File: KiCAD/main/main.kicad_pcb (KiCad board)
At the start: 2 copper layers, 21.9 x 63.9 mm, 45 parts, among them J1 USB_C_Receptacle_USB2.0_14P, J2 Conn_Coaxial, J3 Conn_01x07_Socket, SW1 SW_SPDT, U1 SX1262IMLTRT, U2 TP4056-42-ESOP8, U3 BGS12P2L, U4 ESP32-S3-MINI-1, U6 MIC5219-3.3YMM, U7 CH340X

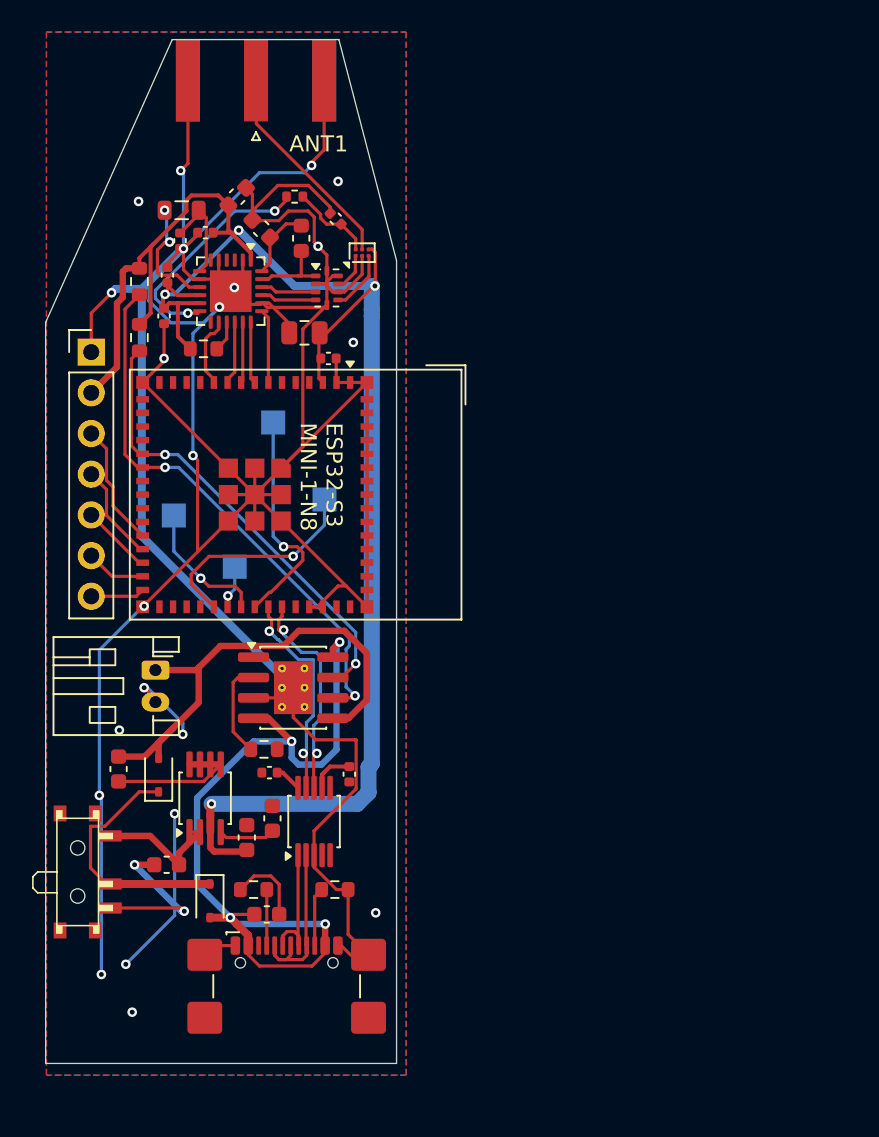
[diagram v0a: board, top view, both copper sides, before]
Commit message: Rev 3 done!
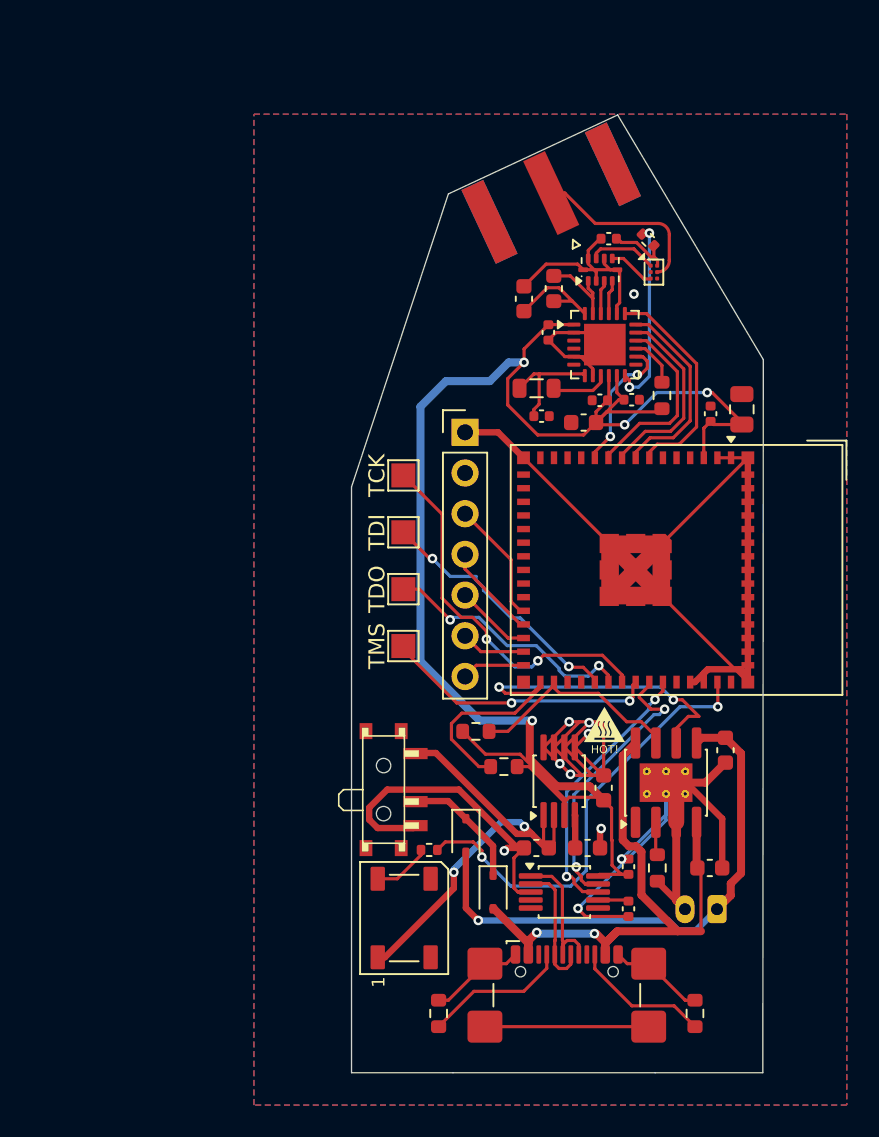
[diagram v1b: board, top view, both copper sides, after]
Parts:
- removed the G*** at (98.8, 76.4)
- removed TP1, TP2, TP3, TP4: TestPoint, TestPoint:TestPoint_Pad_1.5x1.5mm
- added D3: WS2812B, LED_SMD:LED_WS2812B_PLCC4_5.0x5.0mm_P3.2mm, F.Cu at (107.4, 85.3)
- added G***: LOGO, customlib:Hot_Sym, F.Cu at (119.9, 73.2)
- added R18: 450R, Resistor_SMD:R_0402_1005Metric, F.Cu at (108.9, 81.1)
- added TCK: TestPoint, TestPoint:TestPoint_Pad_1.5x1.5mm, F.Cu at (107.3, 57.7)
- added TDI: TestPoint, TestPoint:TestPoint_Pad_1.5x1.5mm, F.Cu at (107.3, 61.2)
- added TDO: TestPoint, TestPoint:TestPoint_Pad_1.5x1.5mm, F.Cu at (107.3, 64.8)
- added TMS: TestPoint, TestPoint:TestPoint_Pad_1.5x1.5mm, F.Cu at (107.3, 68.3)
- BT1: moved to B.Cu
- moved BT1 38.1 mm to (126.9, 84.8), turned to 180 degrees
- moved C16 37.9 mm to (127.4, 74.8)
- moved R9 37.9 mm to (113.6, 75.9), turned to 0 degrees
- moved R10 32.3 mm to (111.8, 73.7), turned to 180 degrees
- moved C10 29.7 mm to (121.6, 53.0), turned to 0 degrees
- moved R4 28.8 mm to (123.5, 52.7), turned to 90 degrees
- moved C7 28.1 mm to (119.6, 53.0), turned to 180 degrees
- moved C15 27.8 mm to (126.5, 82.2)
- moved C4 27.7 mm to (128.4, 53.6), turned to -90 degrees
- moved C14 25.8 mm to (118.6, 54.4), turned to 0 degrees
- moved R7 25.6 mm to (123.2, 82.2), turned to -90 degrees
- moved C11 25.1 mm to (116.0, 54.0), turned to 180 degrees
- moved L1 24.8 mm to (115.6, 52.3), turned to 0 degrees
- moved U4 24.2 mm to (124.4, 63.6)
- moved C3 24.1 mm to (126.5, 53.9), turned to -90 degrees
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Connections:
- net Net-(SW1-A) renamed +5V
- net V- renamed GND
- C10 pad 1: VCC -> +3.3V
- C14 pad 2: VCC -> +3.3V
- C17 pad 2: VCC -> +3.3V
- C18 pad 2: VCC -> +3.3V
- C2 pad 2: VCC -> +3.3V
- C3 pad 2: VCC -> +3.3V
- C4 pad 2: VCC -> +3.3V
- C6 pad 1: VCC -> +3.3V
- C7 pad 1: VCC -> +3.3V
- R10 pad 2: VCC -> +3.3V
- R4 pad 1: VCC -> +3.3V
- R9 pad 2: VCC -> +3.3V
- U1 pad 1: VCC -> +3.3V
- U1 pad 10: VCC -> +3.3V
- U1 pad 11: VCC -> +3.3V
- U3 pad 4: VCC -> +3.3V
- U4 pad 12: unconnected-(U4-IO8-Pad12) -> SDA
- U4 pad 13: unconnected-(U4-IO9-Pad13) -> SCL
- U4 pad 14: unconnected-(U4-IO10-Pad14) -> ENC_PHS_B
- U4 pad 15: unconnected-(U4-IO11-Pad15) -> ENC_PHS_A
- U4 pad 16: unconnected-(U4-IO12-Pad16) -> SEL
- U4 pad 17: unconnected-(U4-IO13-Pad17) -> PWR
- U4 pad 20: ~{CHRG} -> unconnected-(U4-IO16-Pad20)
- U4 pad 21: ~{STDBY} -> unconnected-(U4-IO17-Pad21)
- U4 pad 3: VCC -> +3.3V
- U4 pad 31: unconnected-(U4-IO35-Pad31) -> ~{STDBY}
- U4 pad 32: unconnected-(U4-IO36-Pad32) -> ~{CHRG}
- U4 pad 44: unconnected-(U4-IO46-Pad44) -> NEOPXL_D
- U6 pad 3: VCC -> +3.3V
- U7 pad 10: VCC -> +3.3V
- U7 pad 7: VCC -> +3.3V
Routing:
- net VCC: track 118.4 -> 0.00 mm, vias 4 -> 0
- net +3.3V: track 0.00 -> 107.8 mm, vias 0 -> 4
- net GND: track 313.6 -> 210.2 mm, vias 24 -> 10
- net NEOPXL_D: track 0.00 -> 27.8 mm, vias 0 -> 2
- net +5V: track 8.50 -> 29.1 mm, vias 0 -> 2
- net TCK: track 8.40 -> 23.6 mm, vias 1 -> 2
- net ~{CHRG}: track 28.7 -> 13.8 mm, vias 2 -> 0
- net TDO: track 2.69 -> 16.2 mm, vias 1 -> 2
- net V+: track 50.0 -> 39.3 mm, vias 4 -> 2
- net SPI_CS: track 4.62 -> 13.7 mm
- net SPI_CLK: track 3.87 -> 12.4 mm
- net SPI_MISO: track 3.80 -> 12.2 mm
- net SPI_MOSI: track 3.95 -> 12.0 mm
- net Net-(D1-K): track 15.6 -> 7.68 mm
- net Net-(J1-CC1): track 3.50 -> 9.12 mm
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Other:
- board size 21.9 x 63.9 mm -> 25.7 x 59.8 mm
- board text added: "This will get VERY hot"
- board text added: "VIP(E)R Rev3.0"
- board text removed: "ANT1"
- board text removed: "ESP32-S3 MINI-1-N8"
- board text removed: "VIP(E)R Rev2.1"
